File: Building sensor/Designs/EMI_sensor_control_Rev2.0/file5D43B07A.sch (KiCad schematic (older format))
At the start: 46 parts, among them U8 AD8021ARZ, U9 AD7763BSVZ

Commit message: overdue backup
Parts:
- removed C17, C25, C26, C27, C28, C29, C30, C31, C33, C34: C 100n, Capacitor_SMD:C_0603_1608Metric_Pad1.05x0.95mm_HandSolder, symbol Device:C
- removed C18: C 33p, Capacitor_SMD:C_0402_1005Metric, symbol Device:C
- removed C19: C 100u, Capacitor_Tantalum_SMD:CP_EIA-7343-30_AVX-N_Pad2.25x2.55mm_HandSolder, symbol Device:C
- removed C21, C32: C 10n, Capacitor_SMD:C_0805_2012Metric_Pad1.15x1.40mm_HandSolder, symbol Device:C
- removed FB1, FB10, FB2, FB3, FB4, FB5, FB6, FB7, FB8, FB9: Ferrite_Bead, Capacitor_SMD:C_0603_1608Metric_Pad1.05x0.95mm_HandSolder, symbol Device:Ferrite_Bead
- removed L2: L 8.2n, Inductor_SMD:L_0603_1608Metric_Pad1.05x0.95mm_HandSolder, symbol Device:L
- removed R18, R65: R 10k, Resistor_SMD:R_1206_3216Metric_Pad1.42x1.75mm_HandSolder, symbol Device:R
- removed R20: R 100, Resistor_SMD:R_1206_3216Metric_Pad1.42x1.75mm_HandSolder, symbol Device:R
- removed R21: R 160k, Resistor_SMD:R_1206_3216Metric_Pad1.42x1.75mm_HandSolder, symbol Device:R
- removed R22, R30: R 10, Resistor_SMD:R_1206_3216Metric_Pad1.42x1.75mm_HandSolder, symbol Device:R
- removed R24, R25: R 18, Resistor_SMD:R_0805_2012Metric_Pad1.15x1.40mm_HandSolder, symbol Device:R
- removed U9: AD7763BSVZ, footprints:AD7763BSVZ, symbol 2019-07-11_15-43-26:AD7763BSVZ
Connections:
- net labels removed: +2V5, ADCReset, ADCSync, ADR0b, ADR1b, ADR2b, AGND1b, AGND2b, AGND3b, AGND4b, DRDY, FSI, FSOb, GNDD, GNDREF, GNDS, MCLK, Pin12b, Pin14b, Pin15b, Pin24b, Pin27b, Pin33b, Pin41b, Pin44b, Pin4b, Pin63b, Pin6b, SCO, SDI, SDLb, SDO, SH0b, SH1, SH2, Vref4.1
- wire segments 262 -> 51

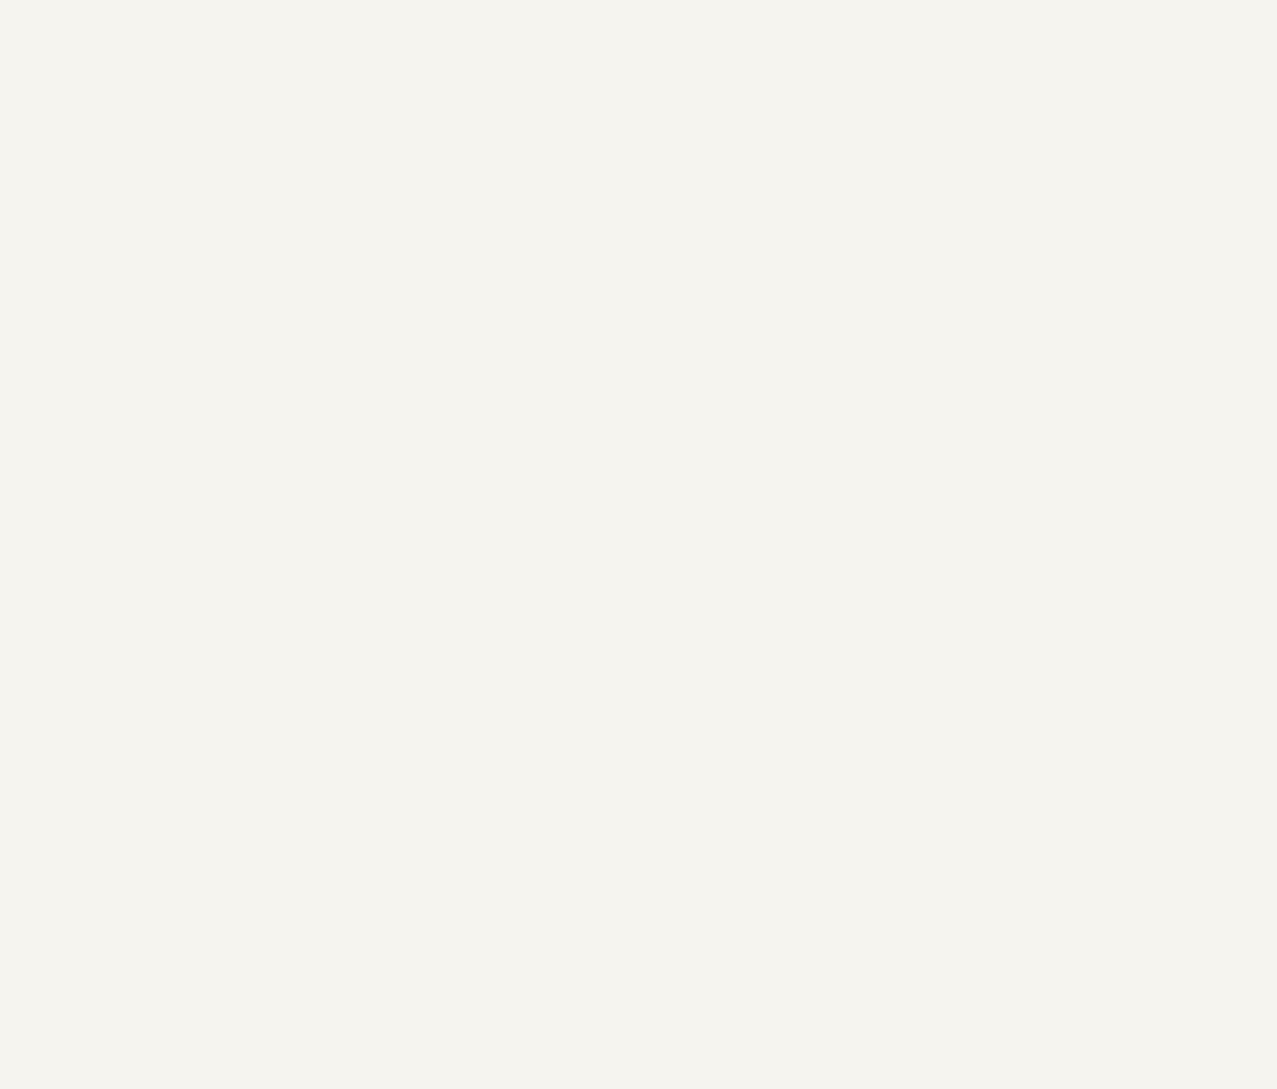
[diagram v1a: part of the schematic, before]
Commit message: backup
2/04/2020
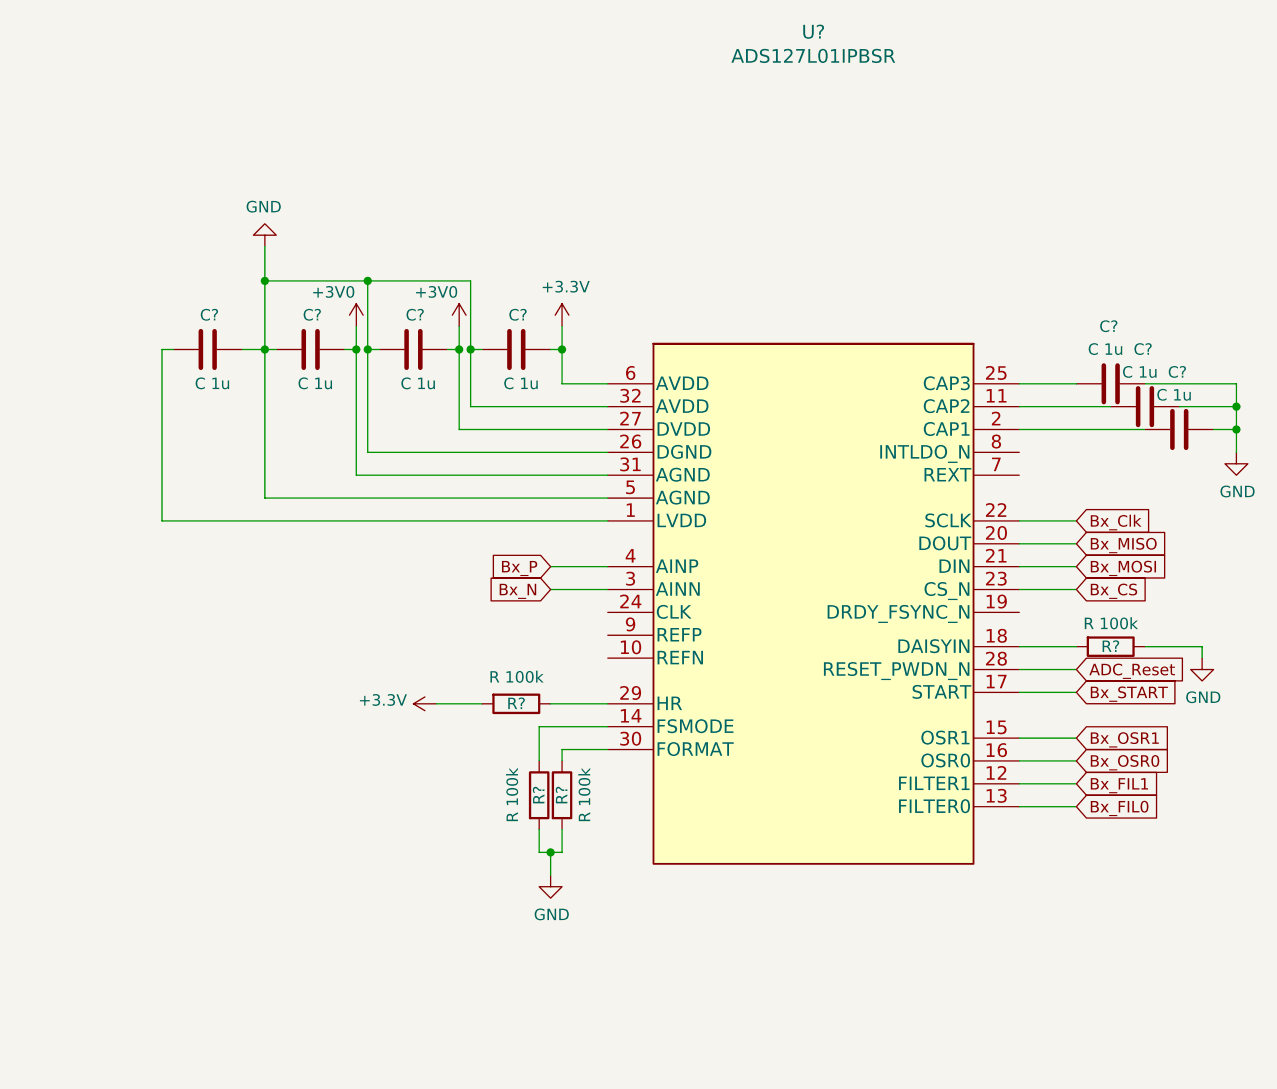
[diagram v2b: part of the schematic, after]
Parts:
- added C? (x7): C 1u, Capacitor_SMD:C_0402_1005Metric, symbol Device:C
- added R? (x4): R 100k, Resistor_SMD:R_0805_2012Metric_Pad1.15x1.40mm_HandSolder, symbol Device:R
- added U?: ADS127L01IPBSR, PBS0032A_N, symbol 2019-12-03_16-41-56:ADS127L01IPBSR
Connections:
- net GND: now also C?.1, C?.1, C?.1, C?.1, C?.1, C?.1, C?.2, R?.1, R?.2, R?.2, U?.26 (DGND), U?.32 (AVDD), U?.5 (AGND)
- new net: C?.1, U?.1 (LVDD)
- new net: R?.2, U?.18 (DAISYIN)
- new net: C?.2, U?.25 (CAP3)
- new net: C?.2, U?.11 (CAP2)
- new net: C?.2, U?.2 (CAP1)
- new net: R?.1, U?.30 (FORMAT)
- new net: R?.1, U?.29 (HR)
- new net: R?.1, U?.14 (FSMODE)
- new net +3V0: C?.2, C?.2, U?.27 (DVDD), U?.31 (AGND)
- new net +3V3: C?.2, R?.2, U?.6 (AVDD)
- new net ADC_Reset: U?.28 (RESET_PWDN_N)
- new net Bx_CS: U?.23 (CS_N)
- new net Bx_Clk: U?.22 (SCLK)
- new net Bx_FIL0: U?.13 (FILTER0)
- new net Bx_FIL1: U?.12 (FILTER1)
- new net Bx_MISO: U?.20 (DOUT)
- new net Bx_MOSI: U?.21 (DIN)
- new net Bx_N: U?.3 (AINN)
- new net Bx_OSR0: U?.16 (OSR0)
- new net Bx_OSR1: U?.15 (OSR1)
- new net Bx_P: U?.4 (AINP)
- new net Bx_START: U?.17 (START)
